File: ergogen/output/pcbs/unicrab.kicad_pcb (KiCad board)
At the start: 2 copper layers, 230 x 104.3 mm, 72 parts

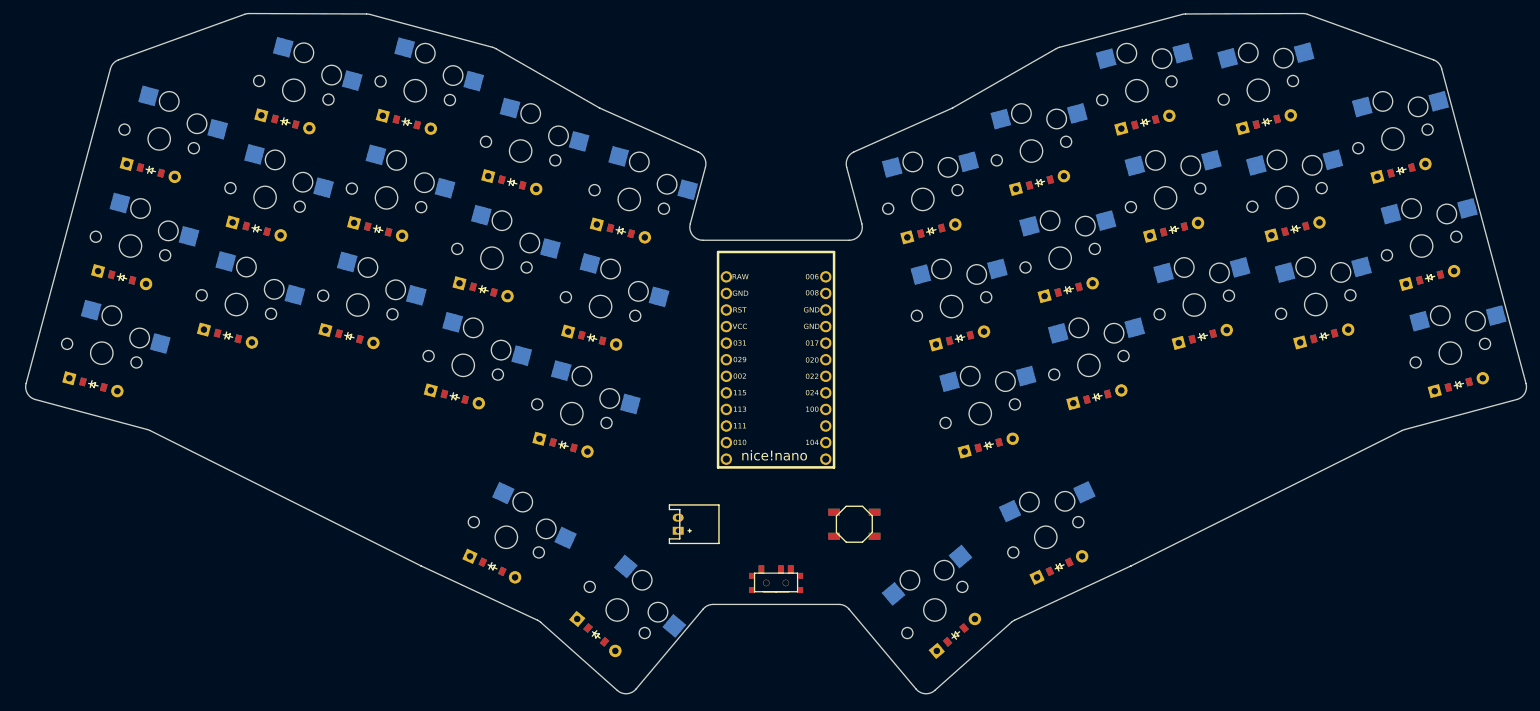
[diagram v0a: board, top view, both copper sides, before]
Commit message: update the kicad file
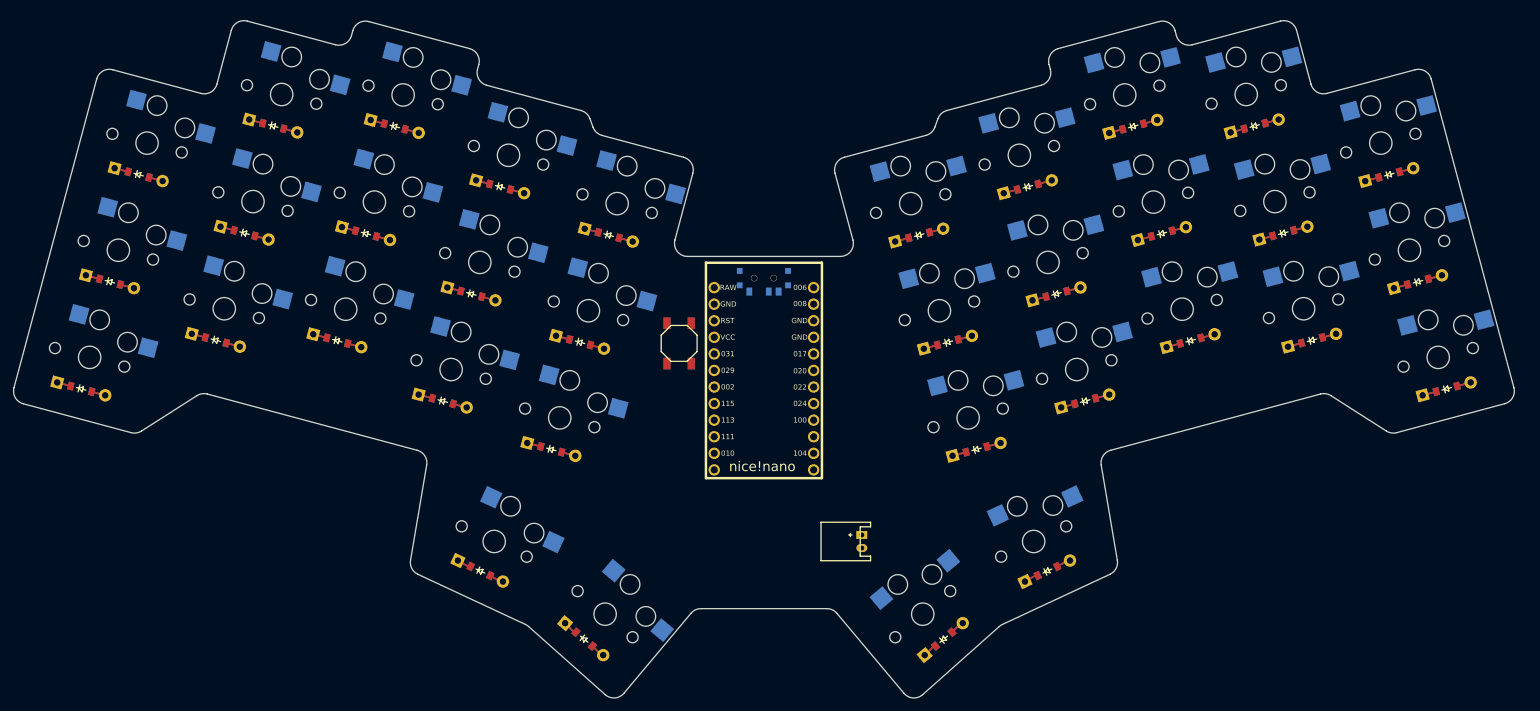
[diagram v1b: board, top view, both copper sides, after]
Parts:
- moved T1 46.8 mm to (172.2, 111.0), turned to 0 degrees
- moved B1 38.6 mm to (159.2, 121.0), turned to 90 degrees
- moved JST1 28.3 mm to (187.2, 151.3), turned to -90 degrees
- moved MCU1 2.48 mm to (172.2, 126.4)
- moved D22 1.97 mm to (251.8, 104.1)
- moved D26 1.97 mm to (228.8, 87.7)
- moved S23 1.97 mm to (246.1, 82.8)
- moved S18 1.97 mm to (275.6, 123.1)
- moved S24 1.97 mm to (236.3, 115.7)
- moved D17 1.97 mm to (144.6, 166.3)
- moved S11 1.97 mm to (128.7, 108.6)
- moved D30 1.97 mm to (204.8, 137.2)
- moved D20 1.97 mm to (268.1, 95.1)
- moved D6 1.97 mm to (97.0, 87.7)
- moved D23 1.97 mm to (247.4, 87.7)
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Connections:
- T1 pad 1: pos -> RAW
- T1 pad 2: RAW -> pos
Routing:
- net P017: track 0.00 -> 21.6 mm
- net P008: track 0.00 -> 21.6 mm
- net P020: track 0.00 -> 21.6 mm
- net P029: track 0.00 -> 21.6 mm
- net P031: track 0.00 -> 21.6 mm
- net P006: track 0.00 -> 21.6 mm
- net P106: track 0.00 -> 8.92 mm
- net P009: track 0.00 -> 8.92 mm
- net mirror_tucky_cluster: track 0.00 -> 4.46 mm
- net mirror_reachy_cluster: track 0.00 -> 4.46 mm
- net tucky_cluster: track 0.00 -> 4.46 mm
- net reachy_cluster: track 0.00 -> 4.46 mm
- net mirror_index_top: track 0.00 -> 4.32 mm
- net mirror_ring_bottom: track 0.00 -> 4.32 mm
- net mirror_ring_home: track 0.00 -> 4.32 mm
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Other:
- board size 230 x 104.3 mm -> 230 x 103.8 mm
- net class Default removed
